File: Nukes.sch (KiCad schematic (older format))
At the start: 21 parts, among them J6 Screw_Terminal_01x02, J7 Screw_Terminal_01x02, J8 Screw_Terminal_01x02, Q4 PMV20ENR, Q5 PMV20ENR, U10 LTV-817S, U9 LTV-817S

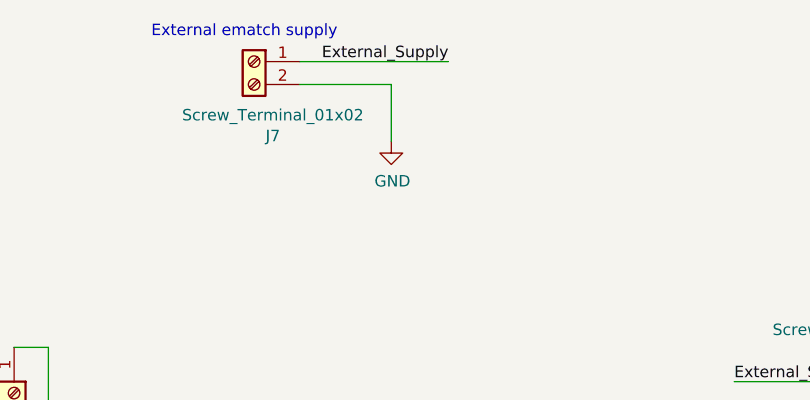
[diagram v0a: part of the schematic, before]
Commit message: shroom
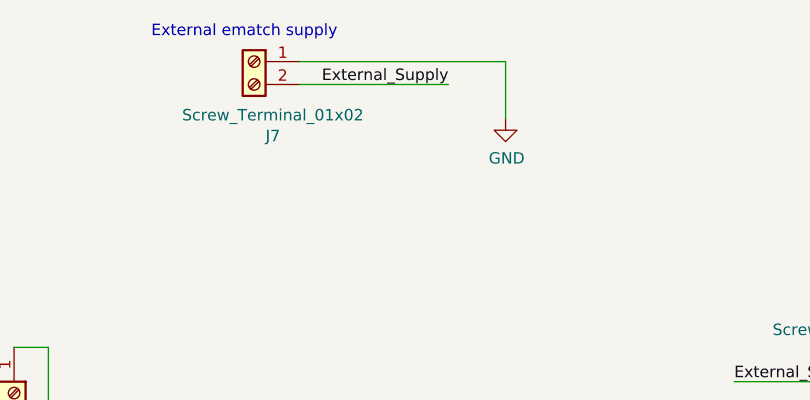
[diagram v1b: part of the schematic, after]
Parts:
- J7: footprint TerminalBlock_Phoenix:TerminalBlock_Phoenix_MPT-0,5-2-2.54_1x02_P2.54mm_Horizontal -> iclr-hw:PHOENIX_1757242
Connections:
- net External_Supply: now also J7.2 (Pin_2); no longer J7.1 (Pin_1)
- net GND: now also J7.1 (Pin_1); no longer J7.2 (Pin_2)
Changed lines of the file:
@@
 F 0 "J7" H 5168 2275 50  0000 C CNN
 F 1 "Screw_Terminal_01x02" H 5168 2366 50  0000 C CNN
-F 2 "TerminalBlock_Phoenix:TerminalBlock_Phoenix_MPT-0,5-2-2.54_1x02_P2.54mm_Horizontal" H 5250 2600 50  0001 C CNN
+F 2 "iclr-hw:PHOENIX_1757242" H 5250 2600 50  0001 C CNN
 F 3 "~" H 5250 2600 50  0001 C CNN
 	1    5250 2600
@@
 Connection ~ 7850 4000
 Wire Wire Line
-	5450 2700 5850 2700
-Wire Wire Line
-	5850 2700 5850 2950
+	6350 2600 6350 2850
 $Comp
 L power:GND #PWR0101
 U 1 1 5DEC1515
-P 5850 2950
-F 0 "#PWR0101" H 5850 2700 50  0001 C CNN
-F 1 "GND" H 5855 2777 50  0000 C CNN
-F 2 "" H 5850 2950 50  0001 C CNN
-F 3 "" H 5850 2950 50  0001 C CNN
-	1    5850 2950
-	1    0    0    -1
-$EndComp
-Text Label 6100 2600 2    50   ~ 0
+P 6350 2850
+F 0 "#PWR0101" H 6350 2600 50  0001 C CNN
+F 1 "GND" H 6355 2677 50  0000 C CNN
+F 2 "" H 6350 2850 50  0001 C CNN
+F 3 "" H 6350 2850 50  0001 C CNN
+	1    6350 2850
+	1    0    0    -1
+$EndComp
+Text Label 6100 2700 2    50   ~ 0
 External_Supply
 Wire Wire Line
-	5450 2600 6100 2600
+	5450 2700 6100 2700
 Text Label 3000 4150 0    50   ~ 0
 External_Supply
@@
 Wire Wire Line
 	4000 3850 4000 4150
+Wire Wire Line
+	5450 2600 6350 2600
 $EndSCHEMATC
